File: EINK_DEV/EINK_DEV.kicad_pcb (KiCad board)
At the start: 2 copper layers, 50.5 x 46.5 mm, 76 parts, among them J1 FPC, J2 Conn_01x06, J3 Conn_01x02, J4 Conn_01x03, J5 Conn_ARM_SWD_TagConnect_TC2030, J6 UART, J7 Conn_Coaxial, J8 GPIO_Header_Dev, P1 USB_C_Plug_USB2.0, Q1 Si1304BDL, SW1 SW_Push, U1 STM32WB55CEU6, U2 TP4056-42-ESOP8, U3 MIC5219-3.3YMM, Y1 32kHz768, Y2 32Mhz

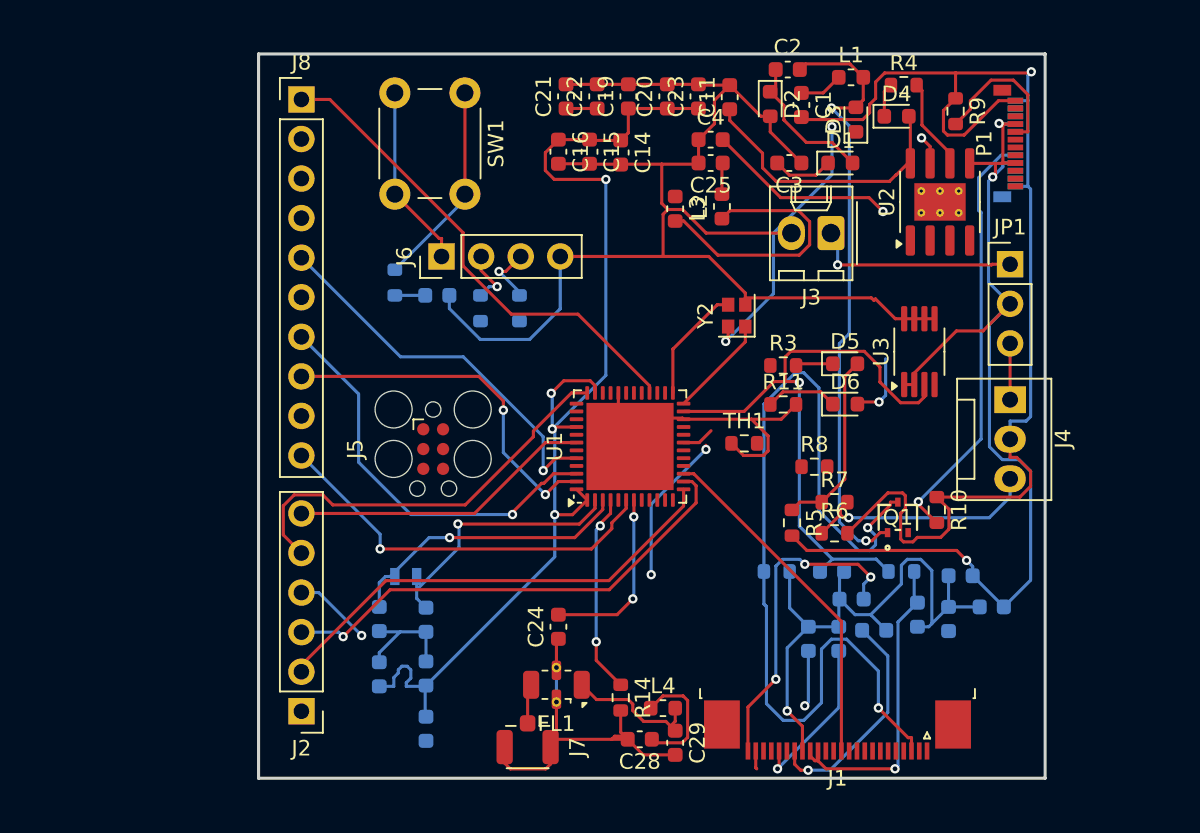
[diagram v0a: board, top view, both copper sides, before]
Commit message: PCB gotowa
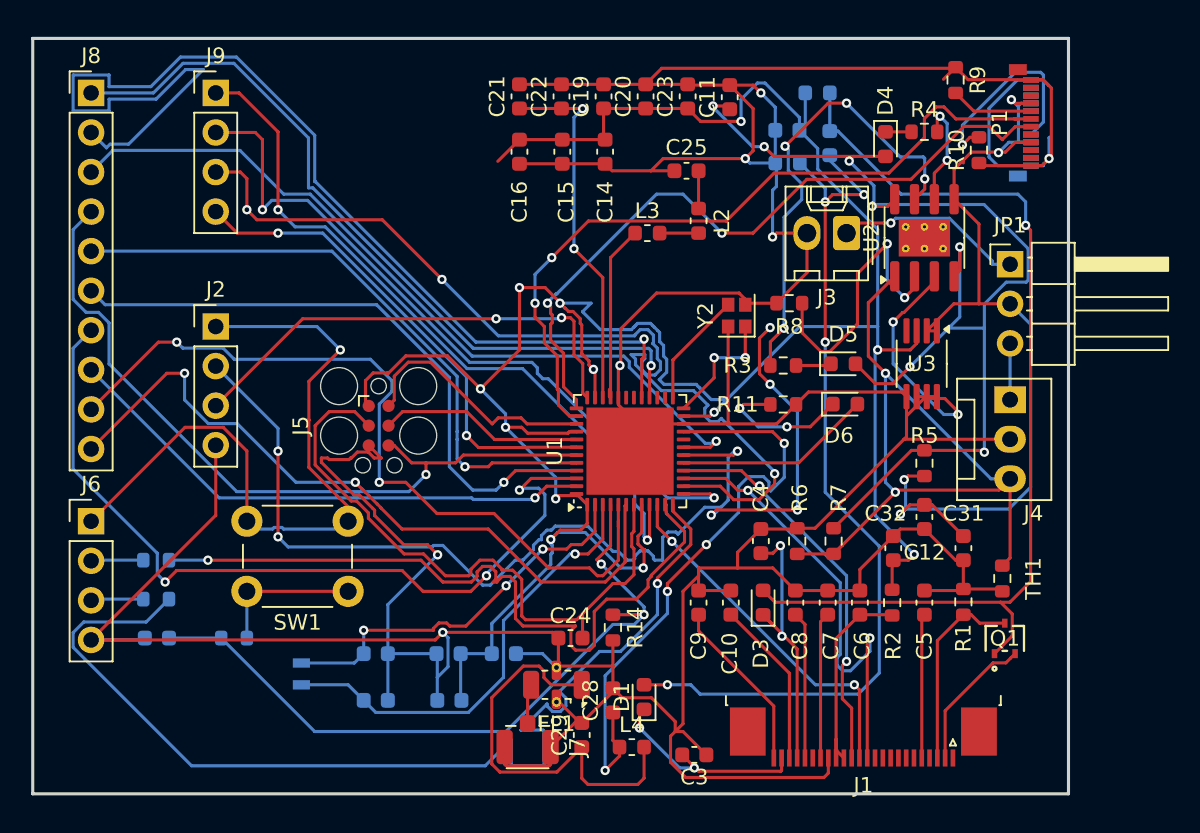
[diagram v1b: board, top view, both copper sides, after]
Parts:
- added J9: USER2, Connector_PinHeader_2.54mm:PinHeader_1x04_P2.54mm_Vertical, F.Cu at (127.5, 72.0)
- C1, C2, D2, L1: moved to B.Cu
- C10, C12, C31, C32, C5, C6, C7, C8, C9, R1, R2: moved to F.Cu
- FL1: value 2,4Ghz LP 50Ohm -> LP
- J2: value Conn_01x06 -> UART1; footprint Connector_PinHeader_2.54mm:PinHeader_1x06_P2.54mm_Vertical -> Connector_PinHeader_2.54mm:PinHeader_1x04_P2.54mm_Vertical
- J6: value UART -> LPUART
- J7: value Conn_Coaxial -> SMD
- J8: value GPIO_Header_Dev -> USER1
- JP1: footprint Connector_PinHeader_2.54mm:PinHeader_1x03_P2.54mm_Vertical -> Connector_PinHeader_2.54mm:PinHeader_1x03_P2.54mm_Horizontal
- Q1: value Si1304BDL -> NMOS
- TH1: value Thermistor_NTC -> THRMST
- moved C3 38.5 mm to (158.2, 114.5)
- moved D1 36.5 mm to (155.0, 110.8), turned to 90 degrees
- moved SW1 32.9 mm to (136.0, 104.0), turned to 180 degrees
- moved D3 31.6 mm to (162.6, 104.7)
- moved R13 29.9 mm to (123.7, 104.5), turned to 0 degrees
- moved C30 28.4 mm to (123.7, 107.0), turned to 180 degrees
- moved J6 28.2 mm to (119.5, 99.5), turned to 0 degrees
- moved R12 26.4 mm to (123.7, 102.0), turned to 0 degrees
- moved C4 26.0 mm to (162.5, 100.8), turned to -90 degrees
- moved J2 25.3 mm to (127.5, 87.0), turned to 0 degrees
- moved R15 25.1 mm to (128.7, 107.0), turned to 0 degrees
- moved R10 23.3 mm to (176.5, 75.7), turned to 90 degrees
- moved TH1 18.7 mm to (178.0, 103.2), turned to 90 degrees
- moved J8 13.5 mm to (119.5, 72.0)
- moved R1 12.1 mm to (175.5, 104.7), turned to 90 degrees
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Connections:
- J2 pad 1: Net-(J2-Pin_1) -> +3.3V
- J2 pad 4: Net-(J2-Pin_4) -> GND
- U1 pad 13: Net-(J2-Pin_2) -> Net-(J9-Pin_2)
- U1 pad 14: Net-(J2-Pin_3) -> Net-(J9-Pin_3)
- U1 pad 18: Net-(J2-Pin_4) -> Net-(J2-Pin_2)
- U1 pad 36: Net-(J2-Pin_5) -> Net-(J2-Pin_3)
- U1 pad 42: Net-(J2-Pin_6) -> Net-(J9-Pin_4)
- U1 pad 9: Net-(J2-Pin_1) -> Net-(J9-Pin_1)
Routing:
- net GND: track 274.2 -> 371.3 mm, vias 4 -> 9
- net Net-(J8-Pin_2): track 0.00 -> 73.5 mm, vias 0 -> 1
- net Net-(U1-PA3): track 0.00 -> 69.4 mm, vias 0 -> 1
- net Net-(J9-Pin_3): track 0.00 -> 60.7 mm, vias 0 -> 3
- net +3V3: track 115.2 -> 172.1 mm, vias 5 -> 12
- net Net-(J8-Pin_9): track 0.00 -> 51.3 mm, vias 0 -> 2
- net Net-(J5-SWO): track 0.00 -> 49.4 mm, vias 0 -> 1
- net Net-(J8-Pin_3): track 2.08 -> 51.0 mm, vias 0 -> 1
- net D+: track 0.00 -> 48.0 mm, vias 0 -> 2
- net Net-(D1-A): track 9.30 -> 56.9 mm, vias 0 -> 4
- net Net-(U1-PA2): track 0.00 -> 47.4 mm, vias 0 -> 1
- net Net-(J9-Pin_2): track 0.00 -> 47.1 mm, vias 0 -> 2
- net RESE: track 59.9 -> 12.8 mm, vias 2 -> 0
- net Net-(J9-Pin_1): track 0.00 -> 46.7 mm, vias 0 -> 2
- net D-: track 0.00 -> 46.5 mm, vias 0 -> 2
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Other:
- board size 50.5 x 46.5 mm -> 66.5 x 48.5 mm
